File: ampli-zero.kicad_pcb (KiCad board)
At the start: 2 copper layers, 100 x 60 mm, 54 parts, among them J1 Conn_01x01, J10 Conn_01x01, J2 Conn_01x01, J3 Conn_01x01, J4 Conn_01x01, J5 Conn_01x01, J6 Conn_01x01, J7 Conn_01x01, J8 Conn_01x01, J9 Conn_01x01, Q10 2SC5200, Q101 2SA1943, Q102 2N5401, Q103 2SD669, Q104 2SB649, Q112 2N5551, Q2 2N5401, Q3 2N5401, Q4 2N5551, Q5 2N5551, Q7 2N5401, Q8 2N5401, Q9 2N5551

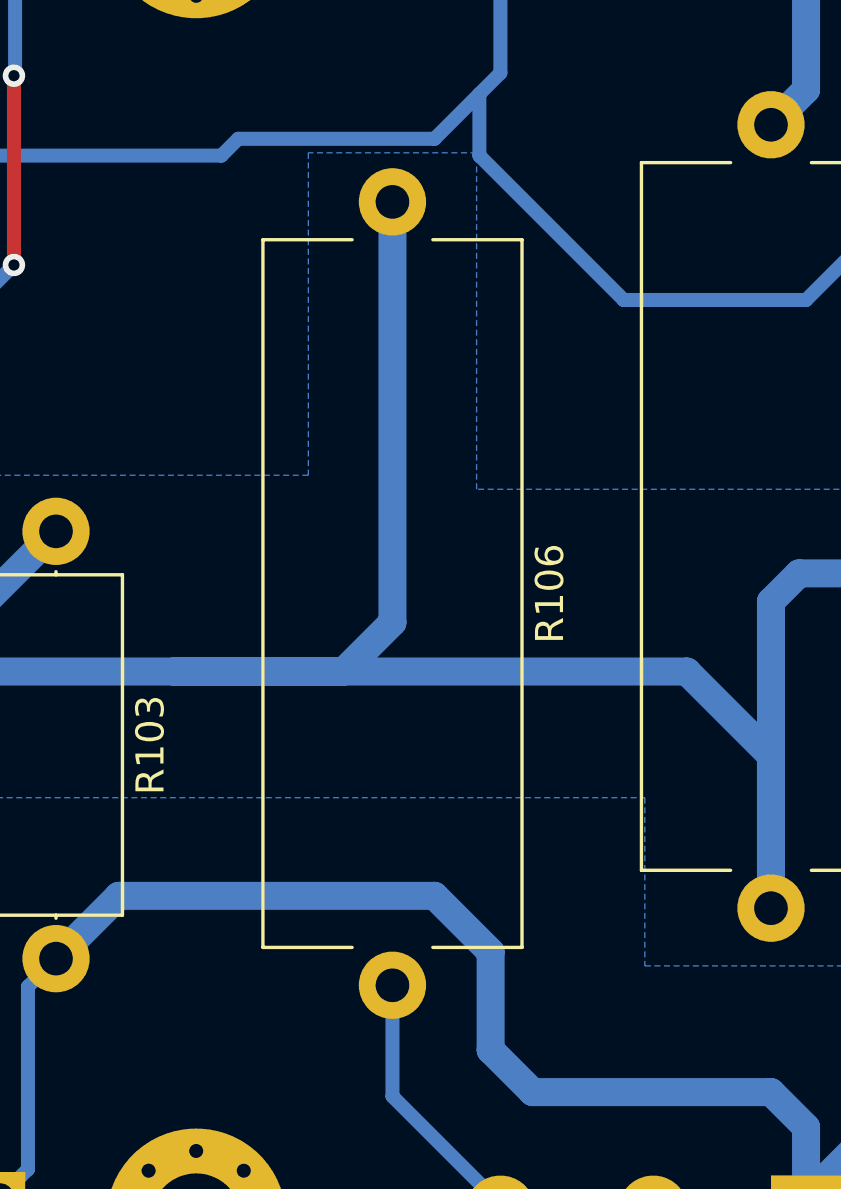
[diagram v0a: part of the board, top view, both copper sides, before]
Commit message: version de 32V
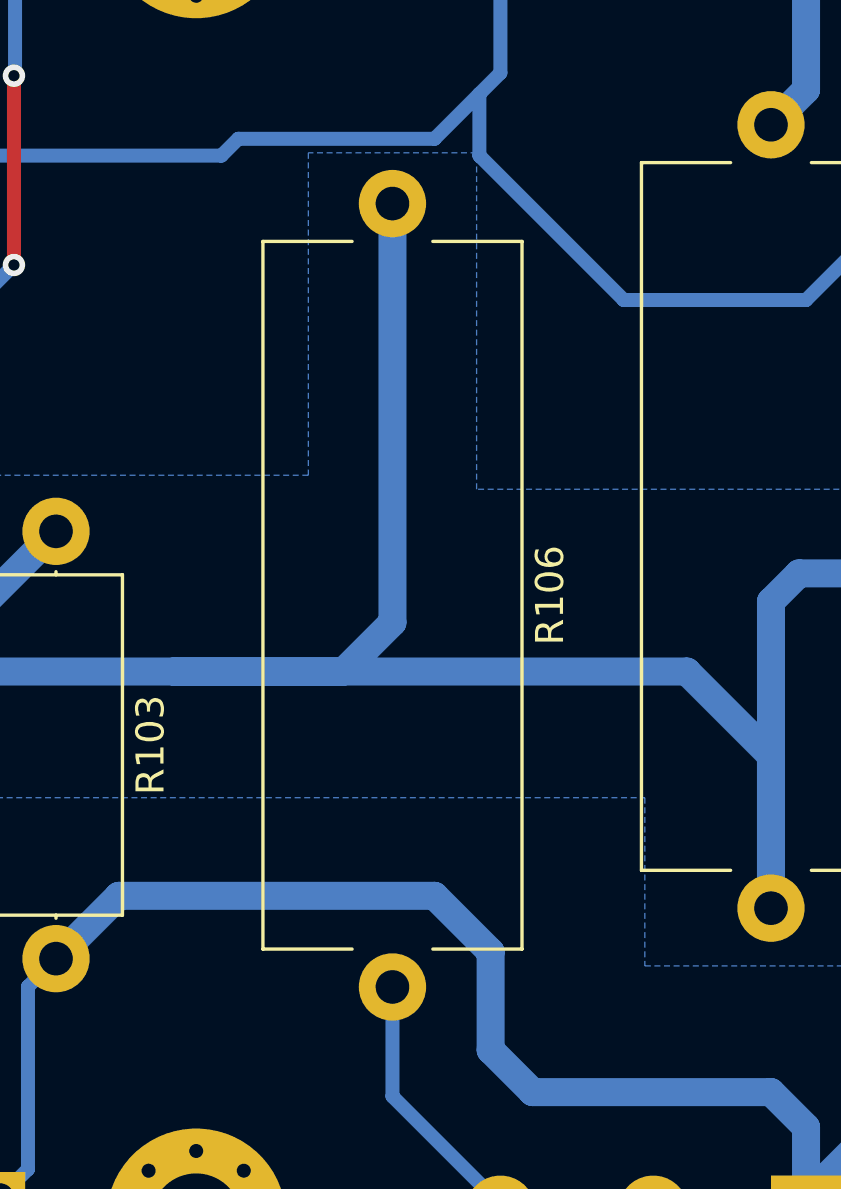
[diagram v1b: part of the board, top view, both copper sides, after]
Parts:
- moved R106 0.06 mm to (200.0, 87.8)
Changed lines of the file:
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@@
     (grid_origin 229 101)
     (pcbplotparams
-      (layerselection 0x00010fc_ffffffff)
+      (layerselection 0x0000030_7ffffffe)
       (plot_on_all_layers_selection 0x0000000_00000000)
       (disableapertmacros false)
@@
       (hpglpendiameter 15.000000)
       (dxfpolygonmode true)
-      (dxfimperialunits true)
+      (dxfimperialunits false)
       (dxfusepcbnewfont true)
       (psnegative false)
@@
       (sketchpadsonfab false)
       (subtractmaskfromsilk false)
-      (outputformat 1)
+      (outputformat 3)
       (mirror false)
-      (drillshape 1)
+      (drillshape 0)
       (scaleselection 1)
       (outputdirectory "")
@@
   )
   (footprint "Resistor_THT:R_Axial_Power_L25.0mm_W9.0mm_P27.94mm" (layer "F.Cu")
-    (at 200 87.75 -90)
+    (at 200 87.81 -90)
     (descr "Resistor, Axial_Power series, Box, pin pitch=27.94mm, 7W, length*width*height=25*9*9mm^3, http://cdn-reichelt.de/documents/datenblatt/B400/5WAXIAL_9WAXIAL_11WAXIAL_17WAXIAL%23YAG.pdf")
     (tags "Resistor Axial_Power series Box pin pitch 27.94mm 7W length 25mm width 9mm height 9mm")
